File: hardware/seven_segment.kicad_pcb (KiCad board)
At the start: 2 copper layers, 95.2 x 50.8 mm, 36 parts, among them J1 Conn_01x16, J2 PJ-102AH, J3 Conn_01x04, SW1 SW_Push, SW2 SW_Push, SW3 SW_Push, U1 STM32F051K8Ux, U10 TPS22810DBVT, U11 STM32F051C8Tx, U12 STM32F051C8Ux, U2 ULN2003A, U3 ULN2003A, U4 AP1117-33, U5 74HC595, U6 74HC595, U7 TPS22810DBVT, U8 TPS22810DBVT, U9 TPS22810DBVT

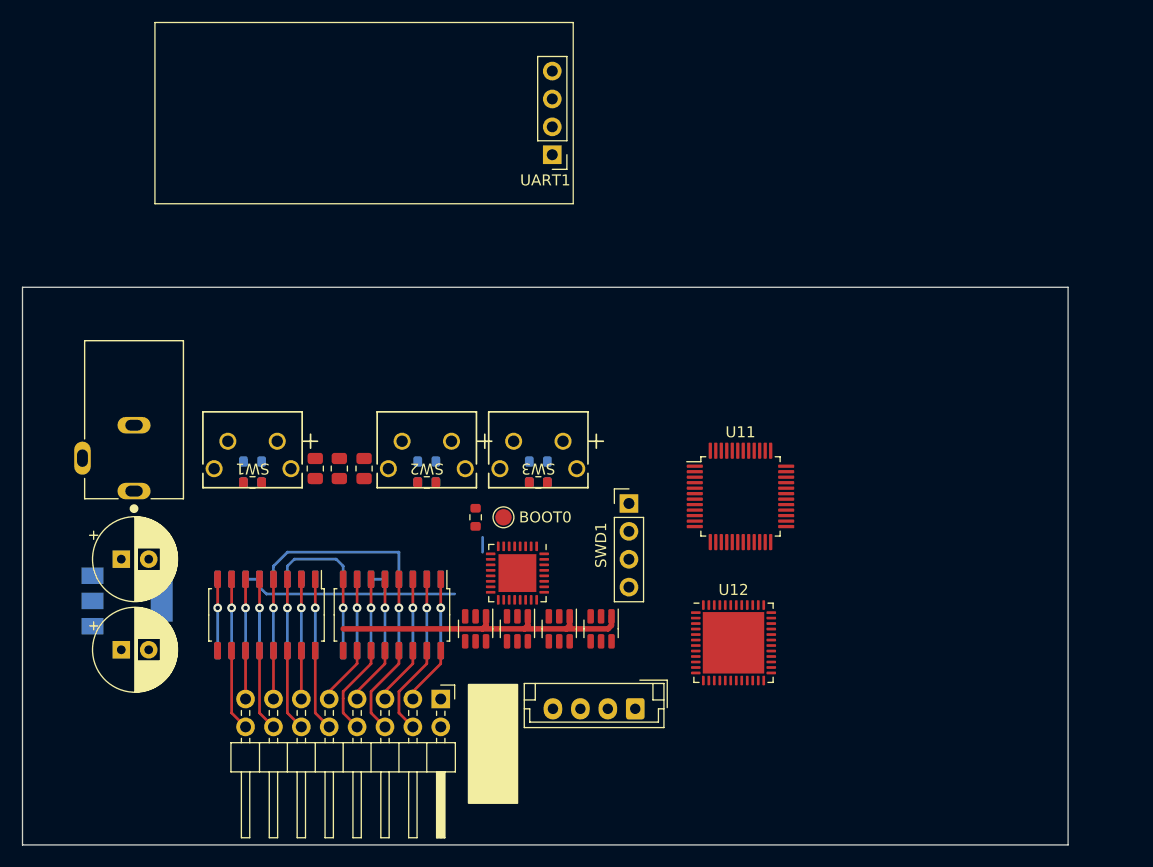
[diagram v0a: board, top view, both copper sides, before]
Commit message: hardware: Version 2
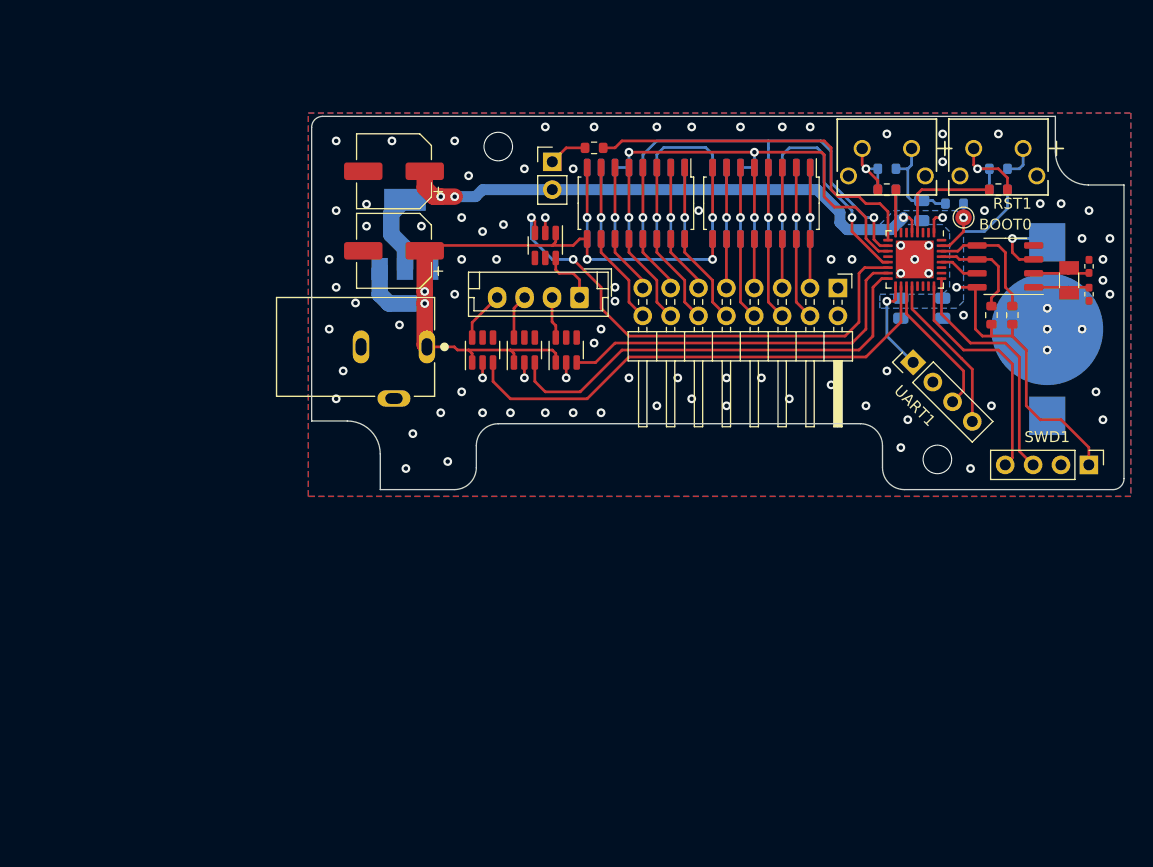
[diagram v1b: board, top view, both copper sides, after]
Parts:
- removed C3: C, Resistor_SMD:R_0603_1608Metric
- removed SW1, SW3: SW_Push, pushbutton:TO_6083716_WRE
- removed U12: STM32F051C8Ux, Package_DFN_QFN:QFN-48-1EP_7x7mm_P0.5mm_EP5.6x5.6mm
- added BT1: Battery_Cell, Battery:BatteryHolder_Keystone_3000_1x12mm, B.Cu at (167.0, 119.4)
- added C10: C, Resistor_SMD:R_0402_1005Metric_Pad0.72x0.64mm_HandSolder, F.Cu at (170.8, 116.2)
- added C4: C, Resistor_SMD:R_0402_1005Metric_Pad0.72x0.64mm_HandSolder, F.Cu at (170.8, 113.7)
- added D1: LED, Connector_PinHeader_2.54mm:PinHeader_1x02_P2.54mm_Vertical, F.Cu at (121.9, 104.1)
- added R7: 10k, Resistor_SMD:R_0603_1608Metric, F.Cu at (125.7, 102.9)
- added RST1: SW_Push, pushbutton:TO_6083716_WRE, F.Cu at (166.1, 105.4)
- added Y1: Crystal, Crystal:Crystal_SMD_3215-2Pin_3.2x1.5mm, F.Cu at (169.0, 114.9)
- C5, C6: footprint Capacitor_THT:CP_Radial_D7.5mm_P2.50mm -> Capacitor_SMD:CP_Elec_6.3x5.9
- C7, C8, C9: moved to B.Cu
- R3: value R -> 10k; moved to F.Cu
- R6: value R -> 10k
- R9: value R -> 10k; moved to B.Cu
- U11: value STM32F051C8Tx -> MCP7940N-xSN; footprint Package_QFP:LQFP-48_7x7mm_P0.5mm -> Package_SO:SO-8_3.9x4.9mm_P1.27mm
- moved C1 73.0 mm to (162.6, 104.8)
- moved R1 73.0 mm to (162.6, 106.7)
- moved R4 73.0 mm to (162.6, 106.7), turned to 0 degrees
- moved C8 59.0 mm to (157.5, 117.5), turned to -90 degrees
- moved C9 58.0 mm to (155.6, 108.6)
- moved R9 52.2 mm to (158.6, 108.0), turned to 0 degrees
- moved J1 52.1 mm to (147.9, 115.6)
- moved C7 51.0 mm to (153.7, 117.5), turned to -90 degrees
- moved C2 50.7 mm to (152.4, 104.8)
- moved U2 50.4 mm to (141.0, 107.9)
- moved U5 50.4 mm to (141.0, 107.9)
- moved U3 50.4 mm to (129.5, 107.9)
- moved U6 50.4 mm to (129.5, 107.9)
- moved C6 50.2 mm to (107.5, 105.0), turned to 180 degrees
- moved BOOT0 50.0 mm to (159.4, 109.2)
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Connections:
- R3 pad 1: Net-(C3-Pad1) -> /SDA
- R6 pad 1: Net-(R6-Pad1) -> /SCL
- R6 pad 2: Net-(C3-Pad1) -> +3V3
- U1 pad 10: unconnected-(U1-Pad10) -> Net-(U1-Pad10)
- U1 pad 14: unconnected-(U1-Pad14) -> Net-(U1-Pad14)
- U1 pad 15: unconnected-(U1-Pad15) -> Net-(U1-Pad15)
- U1 pad 16: unconnected-(U1-Pad16) -> Net-(U1-Pad16)
- U1 pad 28: unconnected-(U1-Pad28) -> Net-(U1-Pad28)
- U1 pad 29: Net-(R5-Pad1) -> /SCL
- U1 pad 30: Net-(R6-Pad1) -> /SDA
- U1 pad 6: Net-(U1-Pad6) -> unconnected-(U1-Pad6)
- U1 pad 7: Net-(U1-Pad7) -> unconnected-(U1-Pad7)
- U1 pad 8: Net-(U1-Pad8) -> Net-(R5-Pad1)
- U10 pad 3: Net-(U1-Pad9) -> Net-(U1-Pad18)
- U11 pad 1: unconnected-(U11-Pad1) -> Net-(C10-Pad1)
- U11 pad 2: unconnected-(U11-Pad2) -> Net-(C4-Pad1)
- U11 pad 3: unconnected-(U11-Pad3) -> Net-(BT1-Pad1)
- U11 pad 4: unconnected-(U11-Pad4) -> GND
- U11 pad 5: unconnected-(U11-Pad5) -> /SDA
- U11 pad 6: unconnected-(U11-Pad6) -> /SCL
- U11 pad 7: unconnected-(U11-Pad7) -> Net-(U1-Pad28)
- U11 pad 8: unconnected-(U11-Pad8) -> +3V3
- U5 pad 13: Net-(U1-Pad18) -> Net-(U1-Pad10)
- U6 pad 13: Net-(U1-Pad18) -> Net-(U1-Pad10)
- U7 pad 3: Net-(U1-Pad6) -> Net-(U1-Pad14)
- U8 pad 3: Net-(U1-Pad7) -> Net-(U1-Pad15)
- U9 pad 3: Net-(U1-Pad8) -> Net-(U1-Pad16)
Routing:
- net +3V3: track 1.34 -> 117.9 mm, vias 0 -> 6
- net Net-(U1-Pad14): track 0.00 -> 45.9 mm, vias 0 -> 2
- net Net-(U1-Pad16): track 0.00 -> 41.2 mm
- net Net-(U1-Pad15): track 0.00 -> 34.3 mm
- net Net-(U1-Pad9): track 0.00 -> 33.7 mm
- net +12V: track 29.2 -> 62.6 mm, vias 0 -> 4
- net Net-(U1-Pad10): track 0.00 -> 33.2 mm, vias 0 -> 1
- net Net-(U1-Pad18): track 15.6 -> 45.7 mm
- net /SWCLK: track 0.00 -> 22.3 mm
- net /SWDIO: track 0.00 -> 21.4 mm
- net GND: track 13.0 -> 31.0 mm, vias 2 -> 93
- net /MOSI: track 0.00 -> 18.0 mm, vias 0 -> 1
- net /UART_RX: track 0.00 -> 14.6 mm
- net /SCK: track 22.6 -> 36.0 mm, vias 0 -> 2
- net /UART_TX: track 0.00 -> 13.1 mm
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- added copper zone on B.Cu, net +3V3
- added copper zone on B.Cu, net GND
- added copper zone on F.Cu, net GND
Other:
- board size 95.2 x 50.8 mm -> 74 x 34 mm
- board text added: "Hammond 1551KBK max.height 10.4mm"
